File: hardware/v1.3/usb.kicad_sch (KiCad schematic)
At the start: 47 parts, among them J3 USB_C_Receptacle_USB2.0_14P, J4 USB_C_Receptacle_USB2.0_14P, J5 USB_C_Receptacle_USB2.0_14P, U1 ECP5-CABGA256, U6 FT231XQ, U7 TPD2EUSB30A, U8 TPD2EUSB30A, U9 TPD2EUSB30A

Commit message: Update to v1.3 board
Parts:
- TP10, TP11, TP12, TP7, TP8, TP9: now left out of the parts list

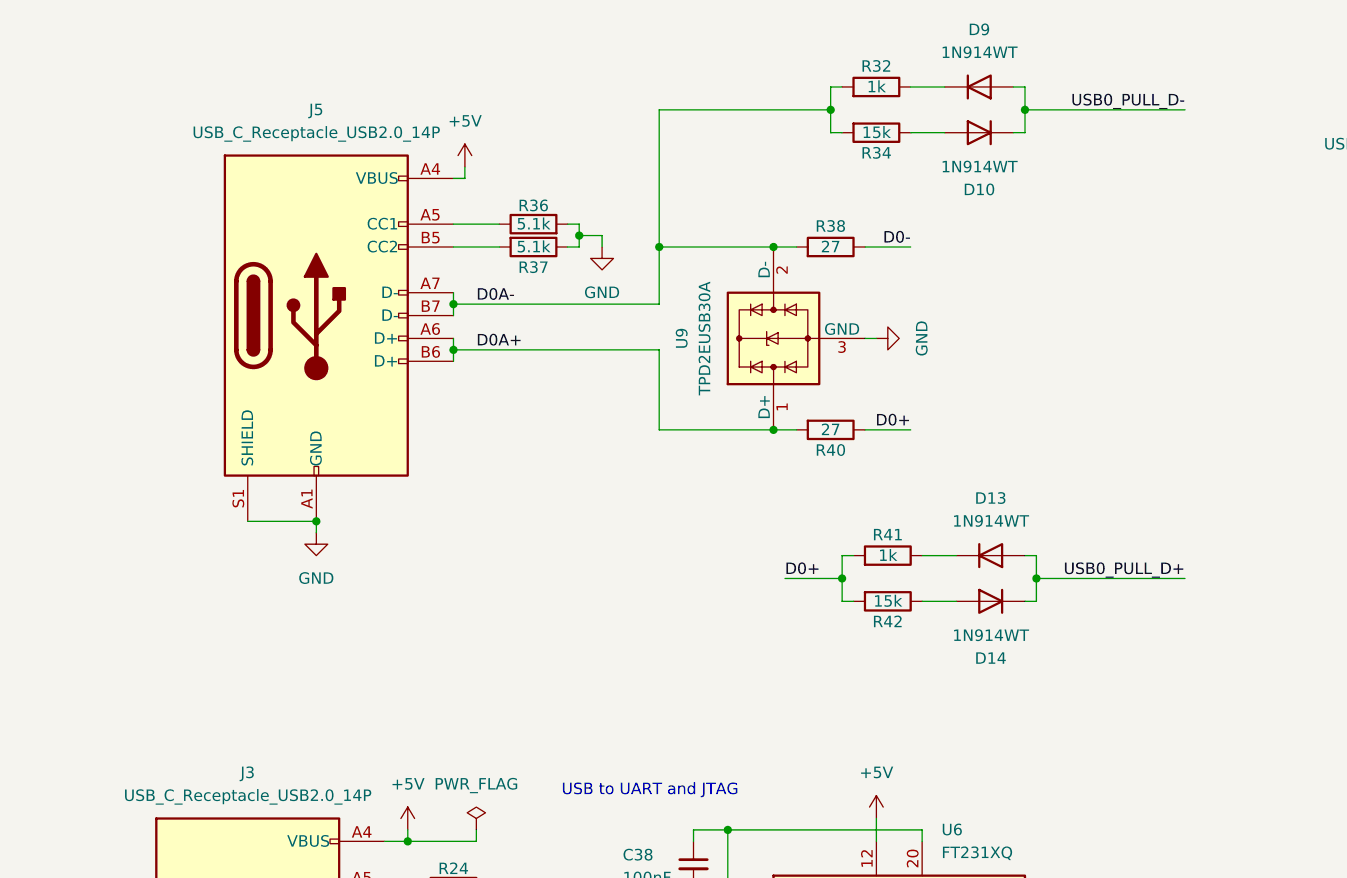
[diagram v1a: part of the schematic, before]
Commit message: Final mass production files
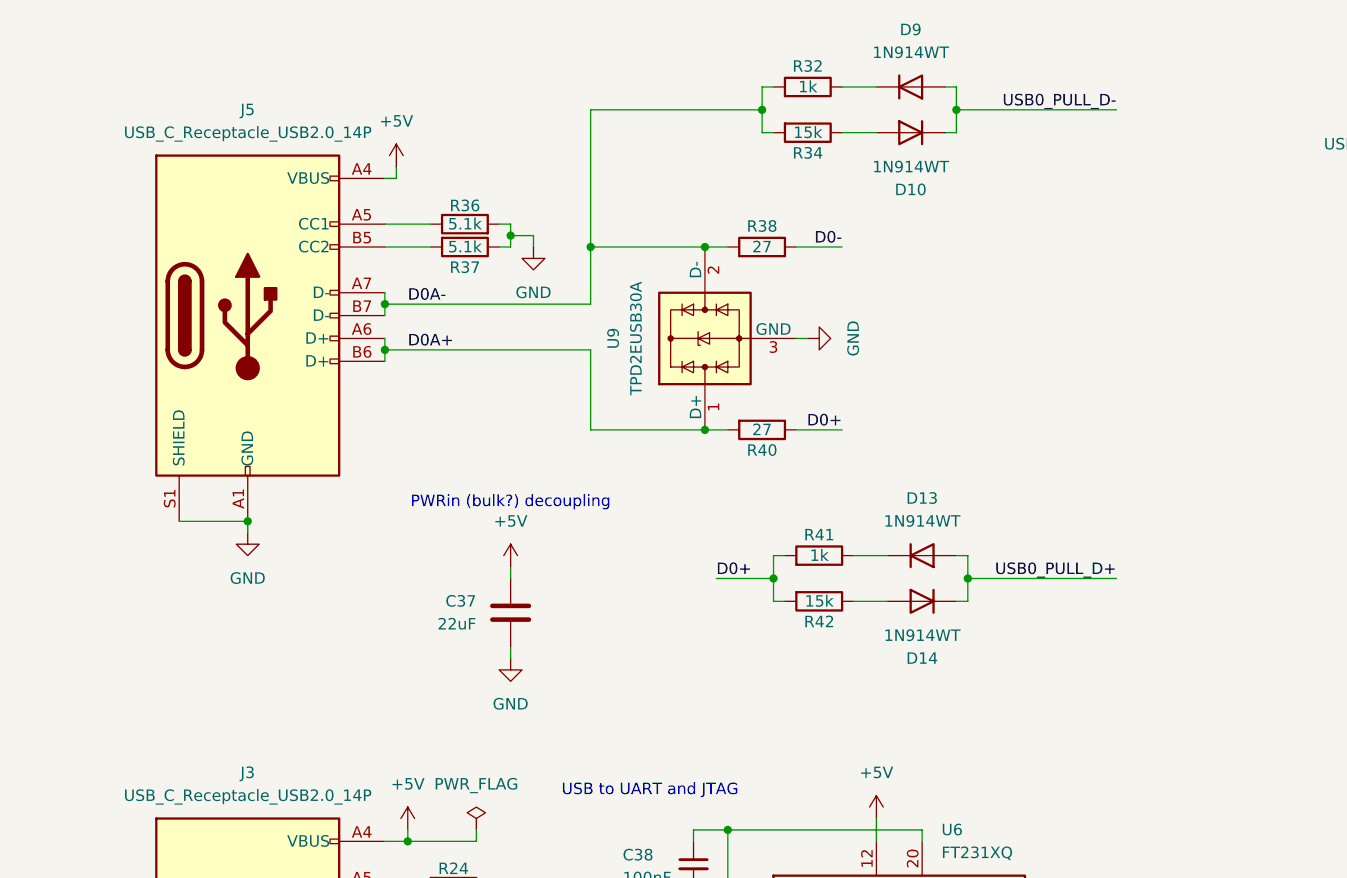
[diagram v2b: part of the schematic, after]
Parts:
- added C37: 22uF, Capacitor_SMD:C_0603_1608Metric, symbol Device:C
- TP10, TP11, TP12, TP9: footprint TestPoint:TestPoint_Pad_D1.0mm -> icepi-lib:TestPoint_Pad_D1.0mm_Blank
- TP7, TP8: footprint TestPoint:TestPoint_Pad_D2.0mm -> icepi-lib:TestPoint_Pad_D2.0mm_Blank
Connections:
- net +5V: now also C37.1
- net GND: now also C37.2
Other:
- note added: "PWRin (bulk?) decoupling"
- moved on the sheet: D10, D13, D14, D9, J5, R32, R34, R36, R37, R38, R40, R41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
